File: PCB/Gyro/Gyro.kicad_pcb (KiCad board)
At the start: 2 copper layers, 70 x 70 mm, 72 parts, among them J1 Reset, J2 TC2030-USB-NL-DS, J3 JST-PH-SM4-TB, J6 USB-C-Socket-V, Q1 CJ2301, SW2 SW_SPST, U1 ESP32-S3-MINI-1, U2 TP4054, U3 ME6211C33M5G-N, U4 MPU-6050

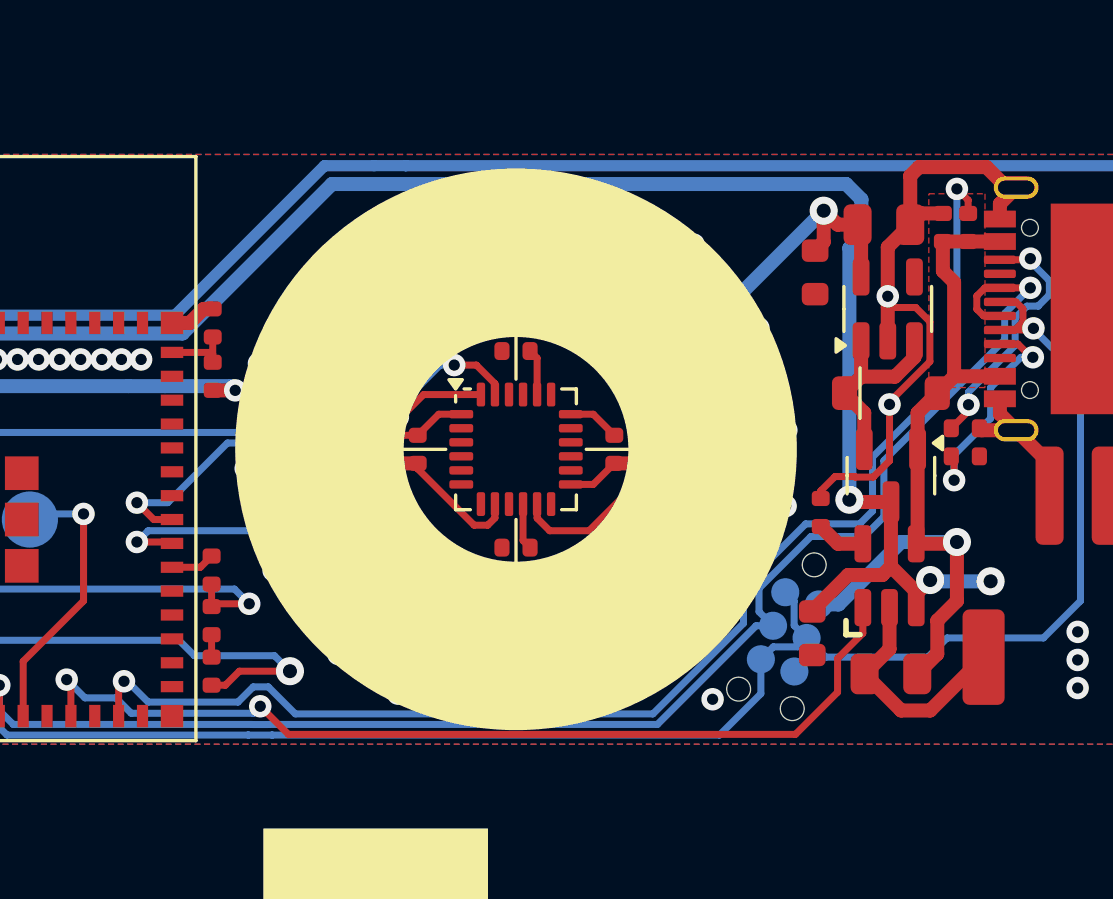
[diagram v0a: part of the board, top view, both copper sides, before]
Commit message: Tweak
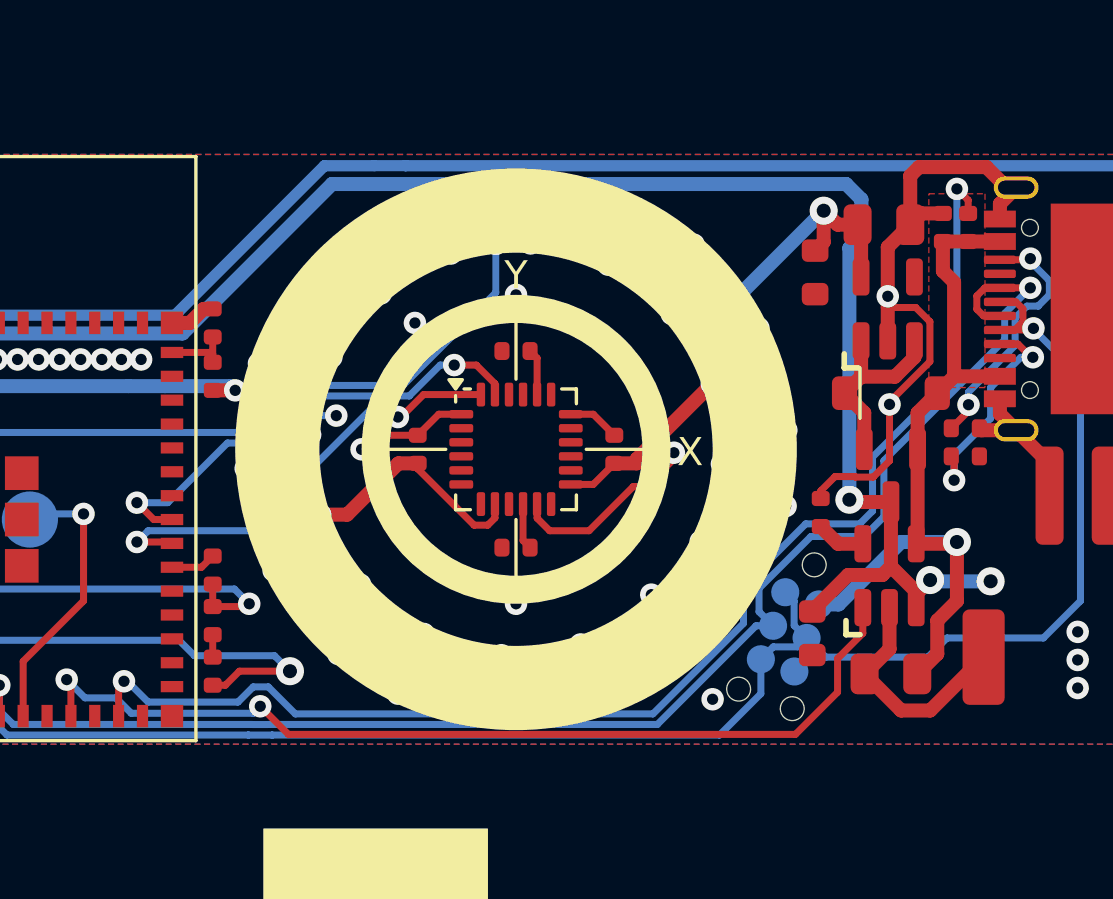
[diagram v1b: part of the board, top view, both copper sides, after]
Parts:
- Q1: footprint Package_TO_SOT_SMD:SOT-23 -> RevK:SOT-23
- U3: footprint Package_TO_SOT_SMD:SOT-23-5 -> RevK:SOT-23-5
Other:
- board text added: "X"
- board text added: "Y"
